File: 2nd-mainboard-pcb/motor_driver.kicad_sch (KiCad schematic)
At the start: 15 parts, among them J11 Servo Motor SM, J12 Stepper Motor, J13 Servo Motor BL Touch, J14 Microstepping, J15 Conn_01x02_Pin, U11 TMC2209_SILENTSTEPSTICK, U12 MPU-6050

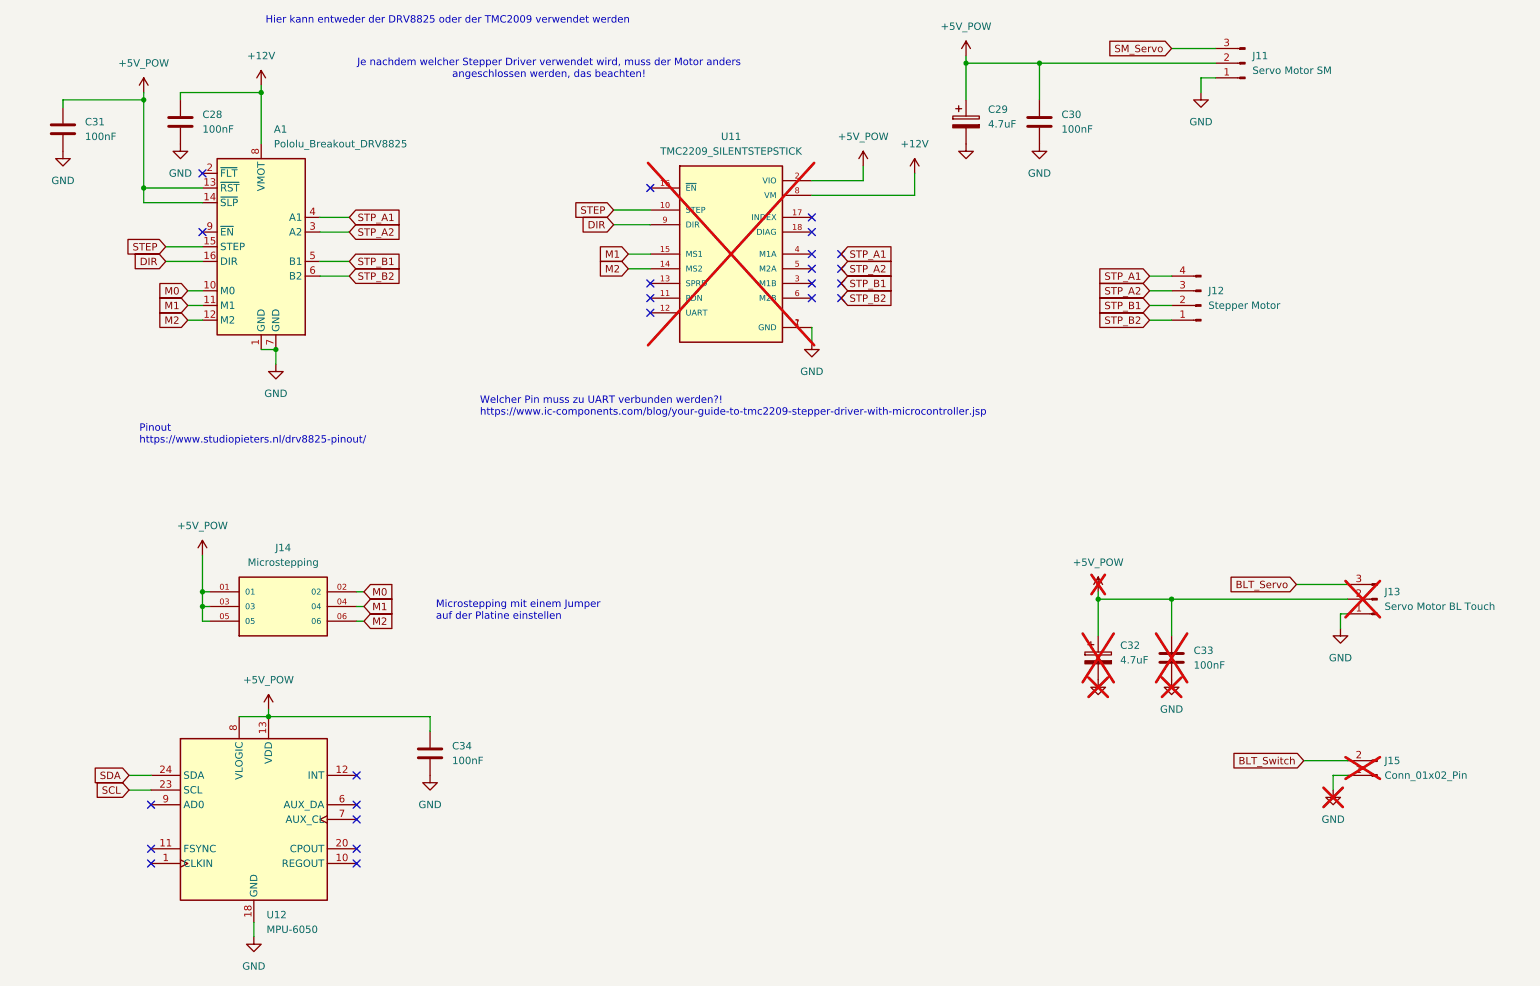
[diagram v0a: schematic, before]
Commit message: mehr positioning
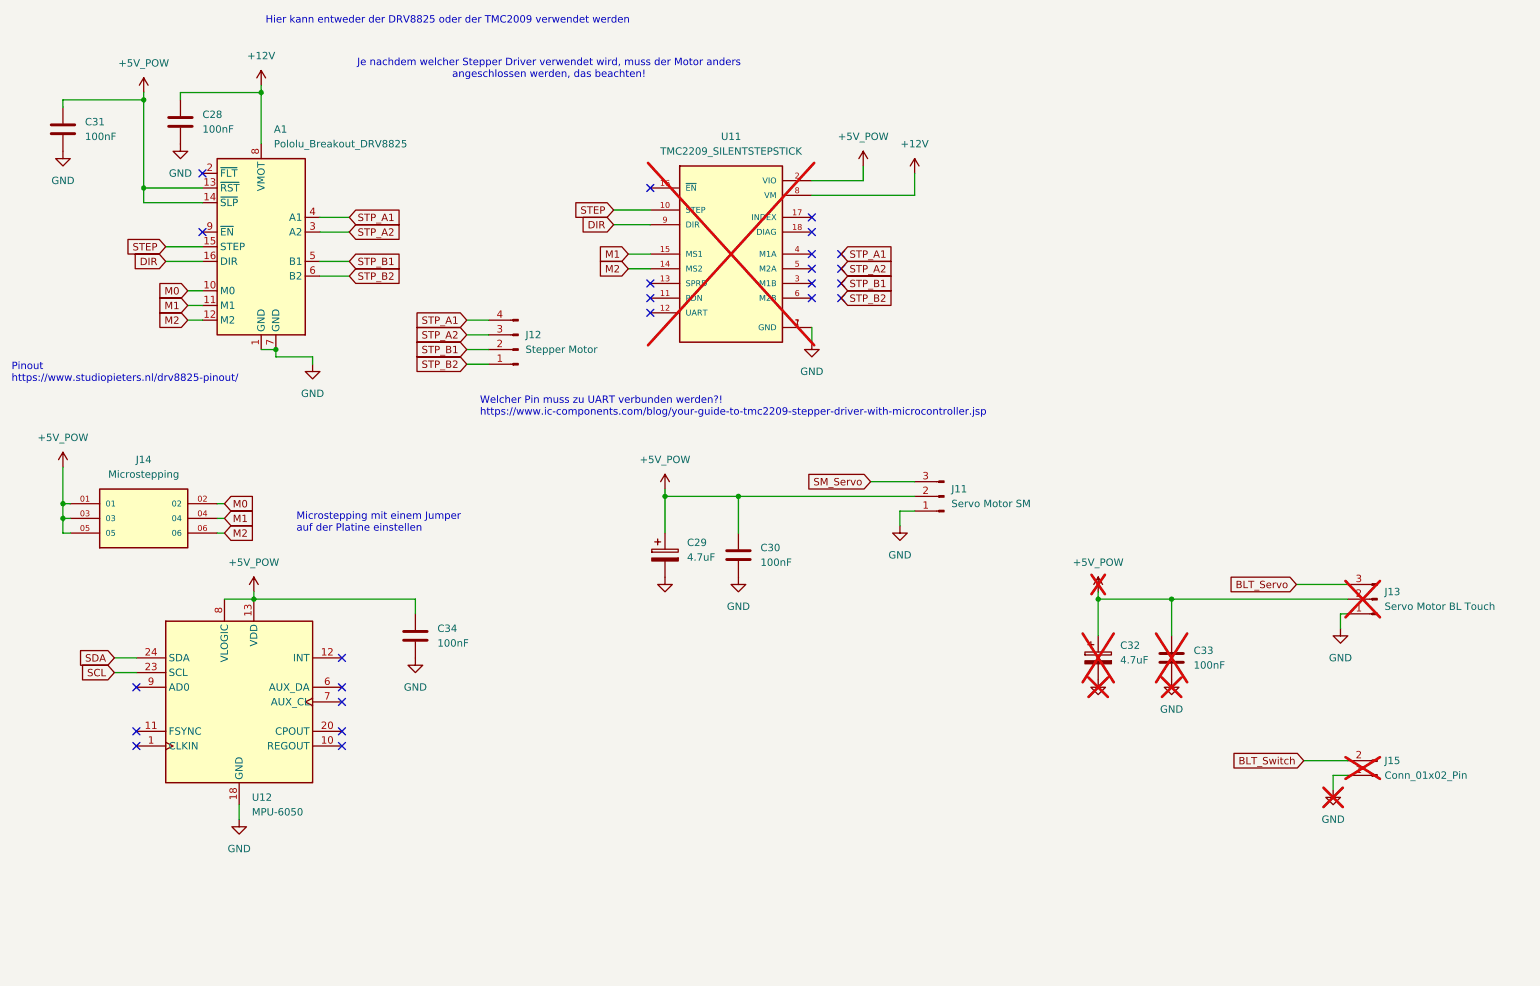
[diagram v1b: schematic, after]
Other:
- moved on the sheet: C29, C30, C34, J11, J12, J14, U12
